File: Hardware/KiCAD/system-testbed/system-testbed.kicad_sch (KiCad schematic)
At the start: 25 parts, among them J1 Stemma QT, J7 Stemma QT, J8 Stemma QT, X1 EYESPI, X11 EYESPI, X6 EYESPI, X7 EYESPI, X8 EYESPI, X9 EYESPI

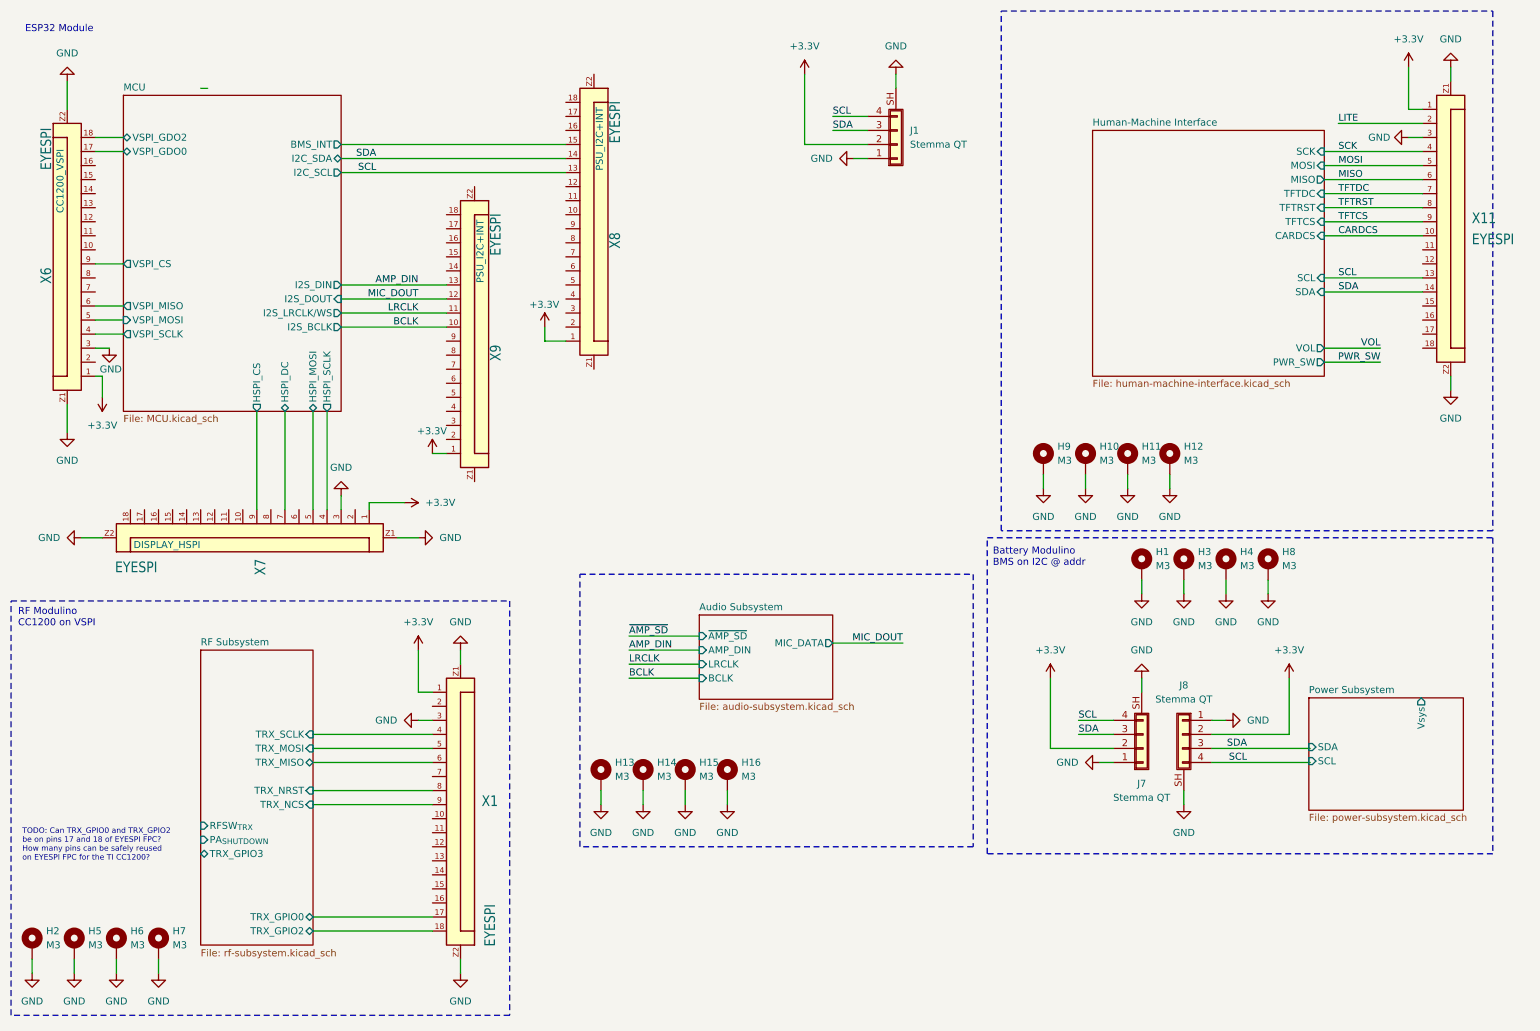
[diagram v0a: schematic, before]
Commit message: feat: update pinouts for mcu #53
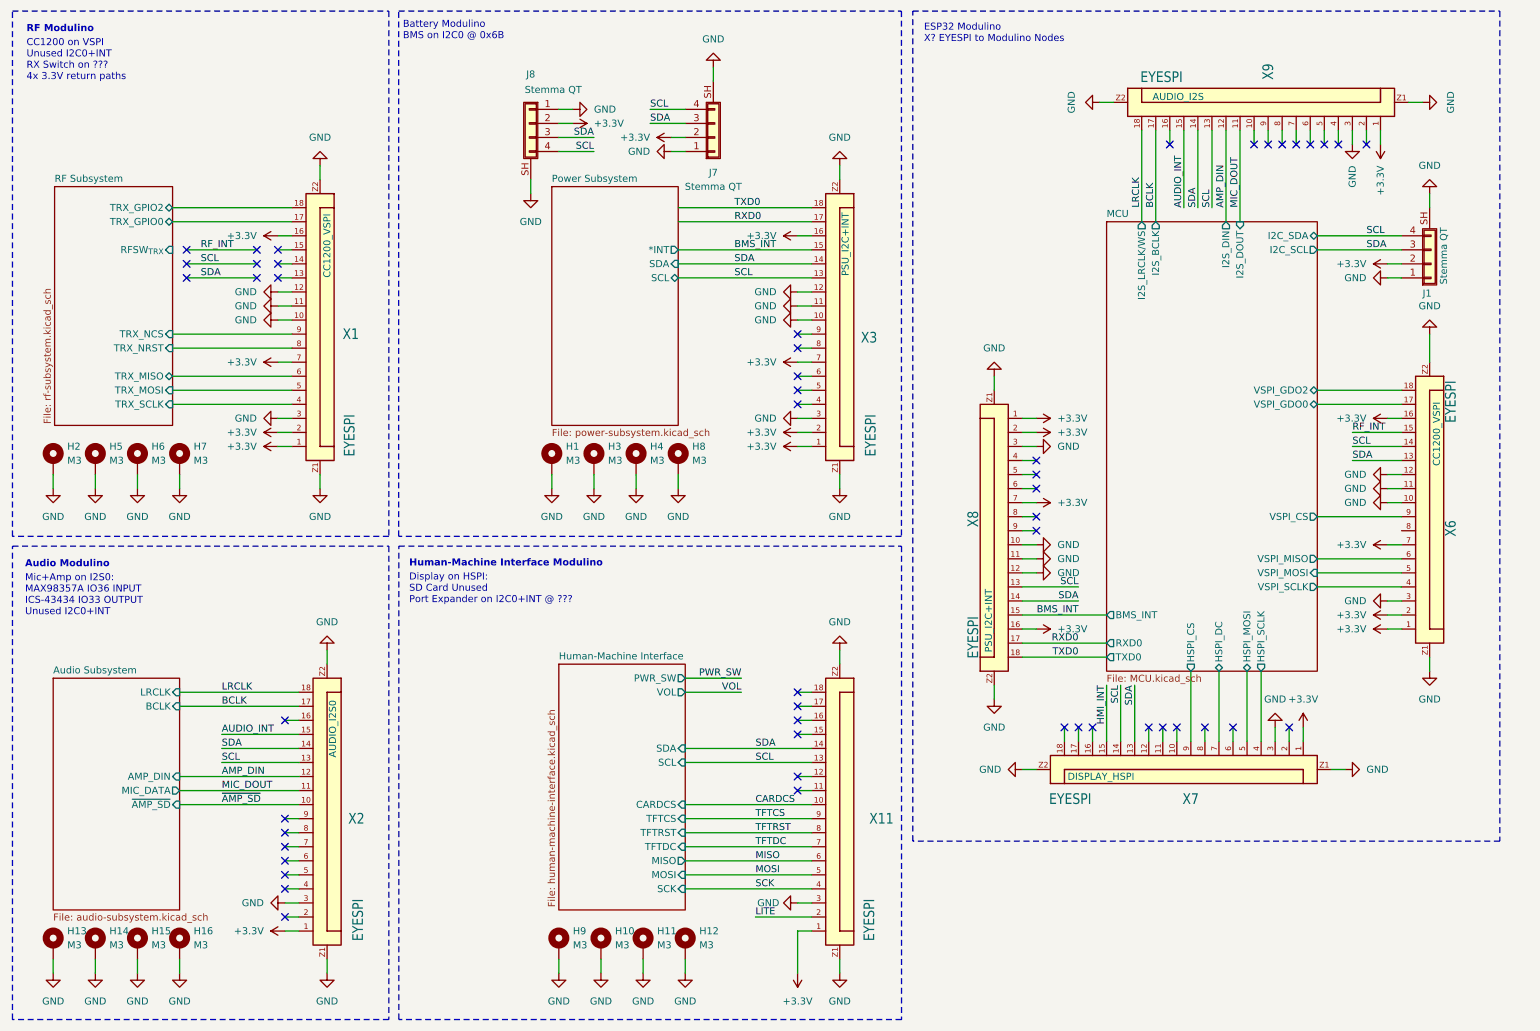
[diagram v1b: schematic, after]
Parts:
- added X2, X3: EYESPI, capstone-project:Adafruit EYESPI FPC Connector, symbol capstone-project:Adafruit EYESPI FPC Connector
- X9: Assignment PSU_I2C+INT -> AUDIO_I2S
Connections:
- net +3.3V: now also X1.16, X1.2, X1.7, X6.16, X6.2, X6.7, X8.16, X8.2, X8.7, X2.1, X3.1, X3.16, X3.2, X3.7
- net AMP_DIN: now also X9.12, X2.12; no longer X9.13
- net BCLK: now also X9.17, X2.17; no longer X9.10
- net GND: now also X1.10, X1.11, X1.12, X6.10, X6.11, X6.12, X8.10, X8.11, X8.12, X8.3, X8.Z1, X8.Z2, X9.3, X9.Z1, X9.Z2, X2.3, X2.Z1, X2.Z2, X3.10, X3.11, X3.12, X3.3, X3.Z1, X3.Z2
- net LRCLK: now also X9.18, X2.18; no longer X9.11
- net MIC_DOUT: now also X9.11, X2.11; no longer X9.12
- net SCL: now also X6.14, X7.14, X9.13, X2.13, X3.13
- net SDA: now also X6.13, X7.13, X9.14, X2.14, X3.14
- net ~{AMP_SD}: now also X2.10
- net AUDIO_INT: now reaches X9.15
- net AUDIO_INT: now also X2.15
- net RXD0: now reaches X8.17
- net RXD0: now also X3.17
- net TXD0: now reaches X8.18
- net TXD0: now also X3.18
- net RF_INT: now reaches X6.15
- net HMI_INT: now reaches X7.15
- net MCU/BMS_INT renamed BMS_INT
- net BMS_INT: now also X3.15
- no-connect marks 0 -> 51
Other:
- sheet MCU ports: added RXD0, TXD0; removed none
- sheet Power Subsystem ports: added *INT; removed Vsys
- sheet RF Subsystem ports: added none; removed PA_{SHUTDOWN}, TRX_GPIO3
- note added: "Audio Modulino"
- note added: "Battery Modulino BMS on I2C0 @ 0x6B"
- note added: "CC1200 on VSPI Unused I2C0+INT RX Switch on ??? 4x 3.3V return paths"
- note added: "Display on HSPI: SD Card Unused Port Expander on I2C0+INT @ ???"
- note added: "ESP32 Modulino X? EYESPI to Modulino Nodes"
- note added: "Human-Machine Interface Modulino"
- note added: "Mic+Amp on I2S0: MAX98357A IO36 INPUT ICS-43434 IO33 OUTPUT Unused I2C0+INT"
- note added: "RF Modulino"
- note removed: "Battery Modulino BMS on I2C @ addr"
- note removed: "ESP32 Module"
- note removed: "RF Modulino CC1200 on VSPI"
- note removed: "TODO: Can TRX_GPIO0 and TRX_GPIO2 be on pins 17 and 18 of EYESPI FPC? How many pins can be safely reused on EYESPI FPC for the TI CC1200?"
- moved on the sheet: H1, H10, H11, H12, H13, H14, H15, H16, H2, H3, H4, H5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
